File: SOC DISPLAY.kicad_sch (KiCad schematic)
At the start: 70 parts, among them IC1 CM BLE, IC2 LM5164QDDATQ1, J2 PRG, J3 OLED, U2 LP2985-3.3, U3 TPS563200, U4 STM32G0B1CBTx, U7 TJA1051T-3

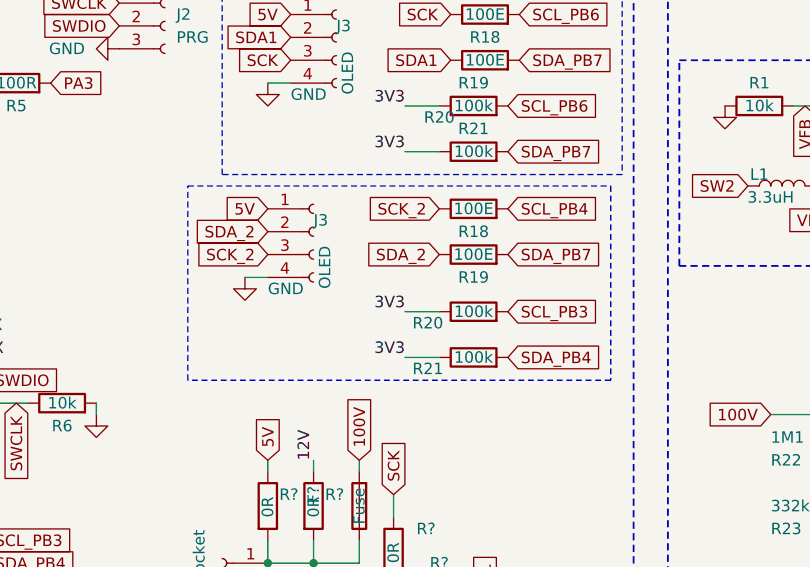
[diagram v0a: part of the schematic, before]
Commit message: Matic
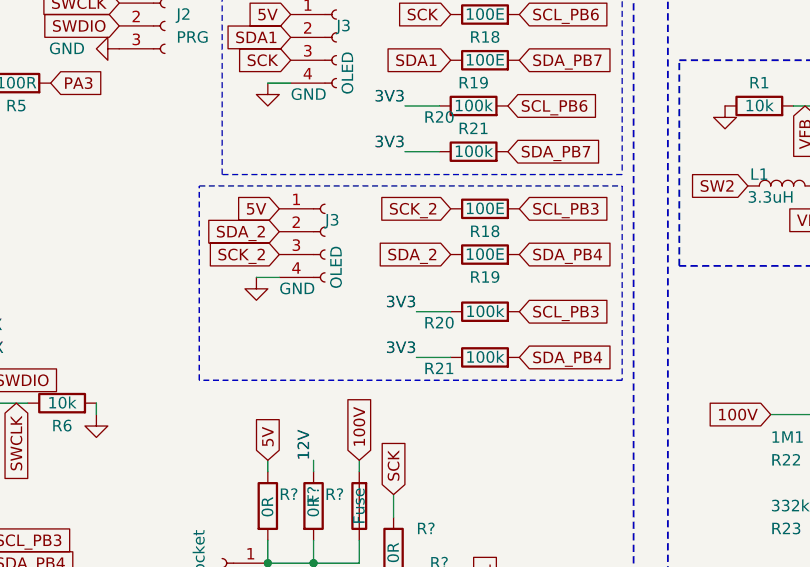
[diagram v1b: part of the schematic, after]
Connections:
- net SCL_PB4 is gone; now on net SCL_PB3: R18.2
- net SDA_PB4: now also R19.2
- net SDA_PB7: no longer R19.2
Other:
- moved on the sheet: J3, R18, R19, R20, R21

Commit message: now
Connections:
- net  SCL_PB3 is gone; now on net SCL_PB3: U4.42 (PB3)
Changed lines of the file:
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@@
     )
   )
-  (global_label " SCL_PB3" (shape input) (at 66.04 80.01 0) (fields_autoplaced)
+  (global_label "SCL_PB3" (shape input) (at 66.04 80.01 0) (fields_autoplaced)
     (effects (font (size 1.27 1.27)) (justify left))
-    (property "Intersheetrefs" "${INTERSHEET_REFS}" (at 78.1381 80.01 0)
+    (property "Intersheetrefs" "${INTERSHEET_REFS}" (at 77.1705 80.01 0)
       (effects (font (size 1.27 1.27)) (justify left) hide)
     )

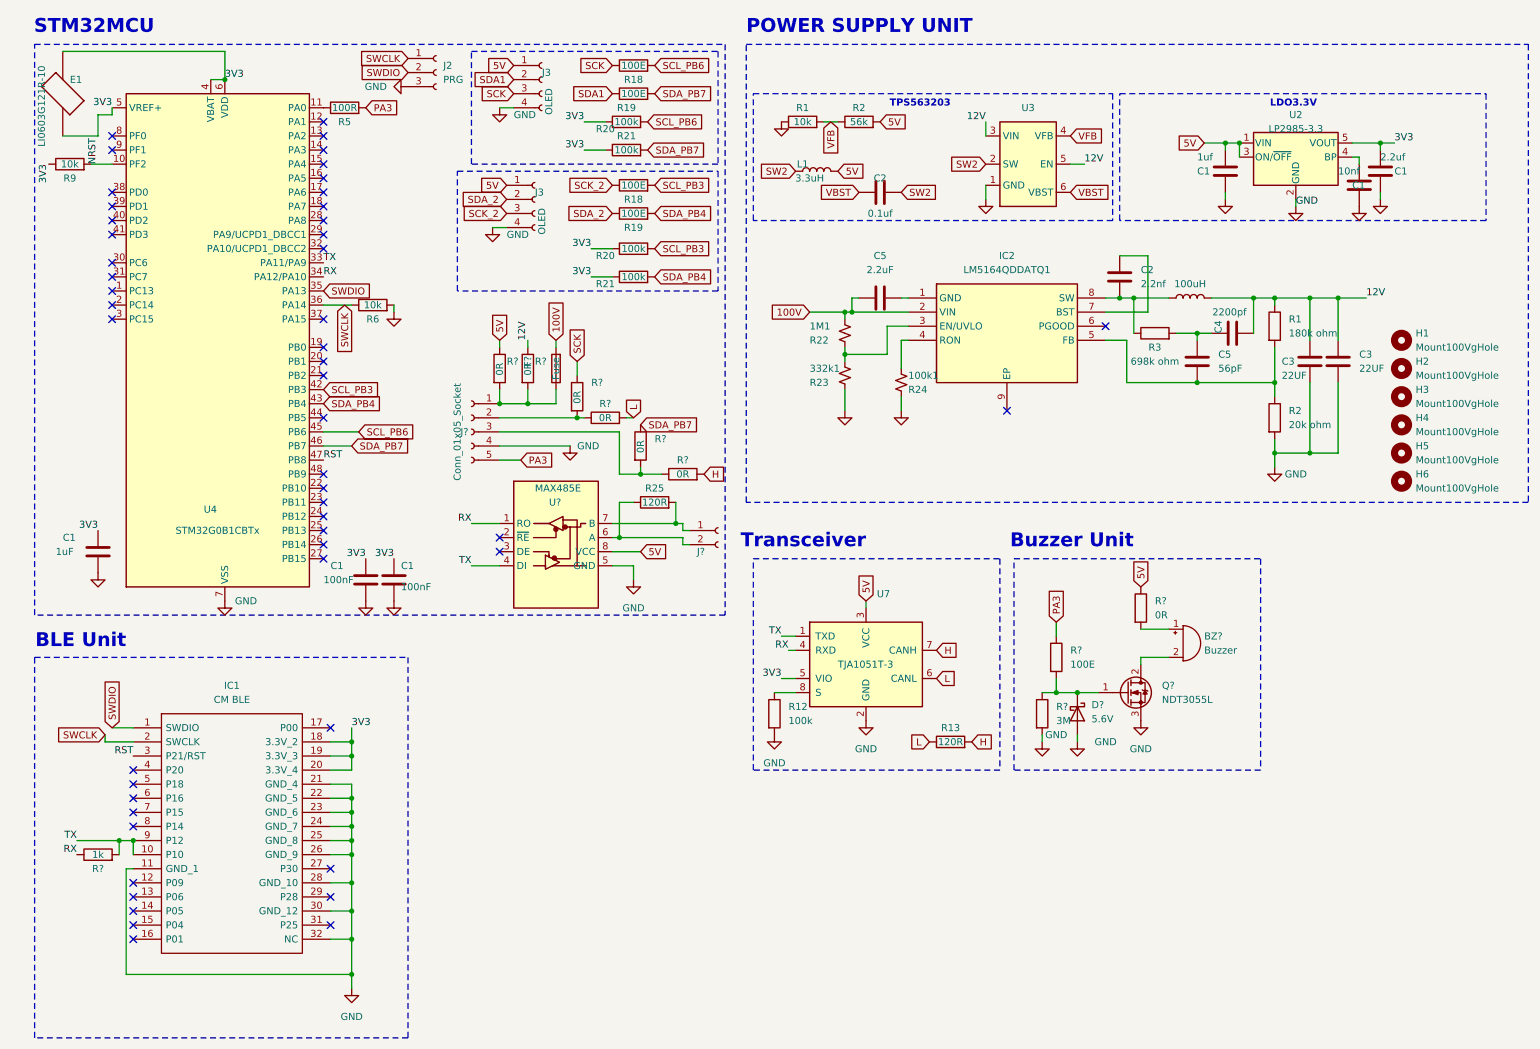
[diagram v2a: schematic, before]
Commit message: Done
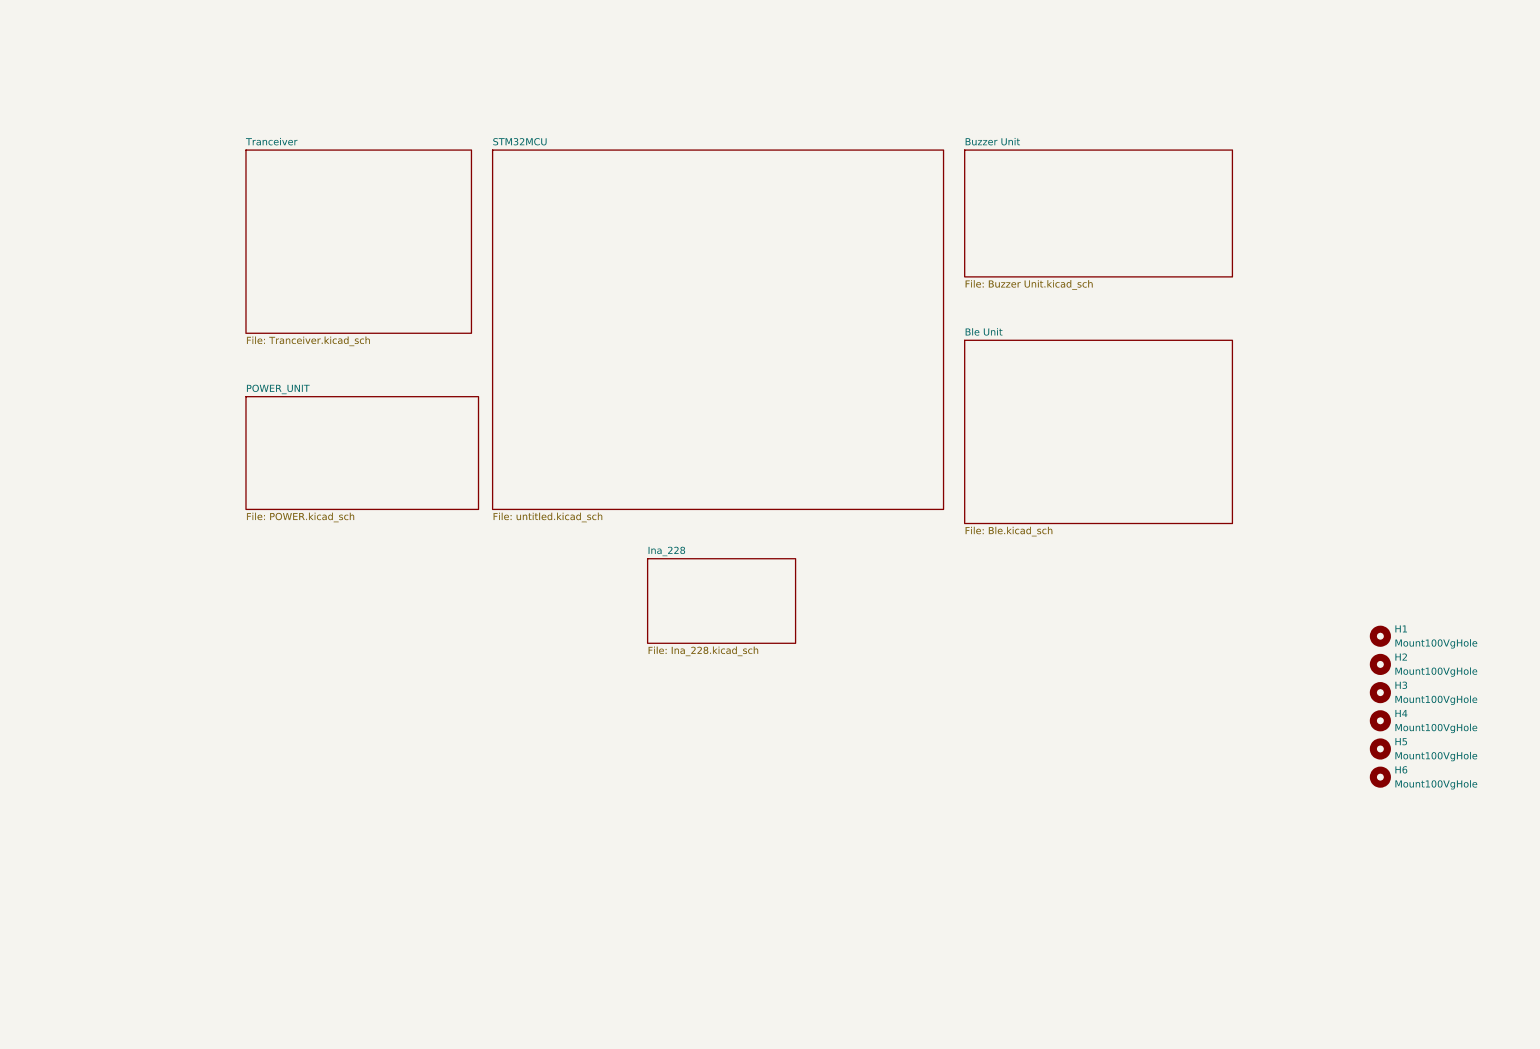
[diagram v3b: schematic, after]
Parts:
- removed 100k1: R24, Resistor_SMD:R_0603_1608Metric_Pad0.98x0.95mm_HandSolder, symbol Device:R_Small_US
- removed 1M1: R22, Resistor_SMD:R_0603_1608Metric_Pad0.98x0.95mm_HandSolder, symbol Device:R_Small_US
- removed 332k1: R23, Resistor_SMD:R_0603_1608Metric_Pad0.98x0.95mm_HandSolder, symbol Device:R_Small_US
- removed BZ?: Buzzer, Buzzer_Beeper:Indicator_PUI_AI-1440-TWT-24V-2-R, symbol Device:Buzzer
- removed C1 (x2): 100nF, Capacitor_SMD:C_0805_2012Metric_Pad1.18x1.45mm_HandSolder, symbol Device:C
- removed C1: 1uf, Capacitor_SMD:C_0805_2012Metric_Pad1.18x1.45mm_HandSolder, symbol Device:C
- removed C1: 1uF, Capacitor_SMD:C_0805_2012Metric_Pad1.18x1.45mm_HandSolder, symbol Device:C
- removed C1: 2.2uf, Capacitor_SMD:C_0805_2012Metric_Pad1.18x1.45mm_HandSolder, symbol Device:C
- removed C1: 10nf, Capacitor_SMD:C_0805_2012Metric_Pad1.18x1.45mm_HandSolder, symbol Device:C
- removed C2: 0.1uf, Capacitor_SMD:C_0805_2012Metric_Pad1.18x1.45mm_HandSolder, symbol Device:C
- removed C2: 2.2nf, Capacitor_SMD:C_0603_1608Metric_Pad1.08x0.95mm_HandSolder, symbol Device:C
- removed C3 (x2): 22UF, Capacitor_SMD:C_1206_3216Metric_Pad1.33x1.80mm_HandSolder, symbol Device:C
- removed C4: 2200pf, Capacitor_SMD:C_0805_2012Metric_Pad1.18x1.45mm_HandSolder, symbol Device:C
- removed C5: 2.2uF, Capacitor_SMD:C_0402_1005Metric_Pad0.74x0.62mm_HandSolder, symbol Device:C
- removed C5: 56pF, Capacitor_SMD:C_0402_1005Metric_Pad0.74x0.62mm_HandSolder, symbol Device:C
- removed D?: 5.6V, Diode_SMD:D_0603_1608Metric_Pad1.05x0.95mm_HandSolder, symbol Device:D_Schottky
- removed E1: LI0603G121R-10, LI0603G121R-10.kicad_mod files:FB_LI0603G121R-10, symbol LI0603G121R-10:LI0603G121R-10
- removed F?: Fuse, Fuse:Fuse_0603_1608Metric_Pad1.05x0.95mm_HandSolder, symbol Device:Fuse
- removed IC1: CM BLE, Library:CM BLE, symbol Library:COMMON_BLUETOOTH
- removed IC2: LM5164QDDATQ1, LIB_LM5164QDDATQ1.kicad_mod files:SOIC127P600X170-9N, symbol LM5164QDDATQ1:LM5164QDDATQ1
- removed J2: PRG, TerminalBlock:TerminalBlock_bornier-3_P5.08mm, symbol Connector:Conn_01x03_Socket
- removed J3 (x2): OLED, TerminalBlock:TerminalBlock_bornier-4_P5.08mm, symbol Connector:Conn_01x04_Socket
- removed J?: Conn_01x05_Socket, Connector_JST:JST_PH_S5B-PH-K_1x05_P2.00mm_Horizontal, symbol Connector:Conn_01x05_Socket
- removed J?: Conn_01x02_Socket, TerminalBlock:TerminalBlock_bornier-2_P5.08mm, symbol Connector:Conn_01x02_Socket
- removed L1: 100uH, Inductor_SMD:L_0805_2012Metric_Pad1.15x1.40mm_HandSolder, symbol Device:L
- removed L1: 3.3uH, Inductor_SMD:L_0402_1005Metric_Pad0.77x0.64mm_HandSolder, symbol Device:L
- removed Q?: NDT3055L, Package_TO_SOT_SMD:SOT-223-3_TabPin2, symbol Transistor_FET:NDT3055L
- removed R1, R6, R9: 10k, Resistor_SMD:R_0603_1608Metric_Pad0.98x0.95mm_HandSolder, symbol Device:R
- removed R1: 180k ohm, Resistor_SMD:R_0603_1608Metric_Pad0.98x0.95mm_HandSolder, symbol Device:R
- removed R12, R20 (x2), R21 (x2): 100k, Resistor_SMD:R_0603_1608Metric_Pad0.98x0.95mm_HandSolder, symbol Device:R
- removed R13, R25: 120R, Resistor_SMD:R_0603_1608Metric_Pad0.98x0.95mm_HandSolder, symbol Device:R
- removed R18 (x2), R19 (x2), R?: 100E, Resistor_SMD:R_0603_1608Metric_Pad0.98x0.95mm_HandSolder, symbol Device:R
- removed R2: 20k ohm, Resistor_SMD:R_0603_1608Metric_Pad0.98x0.95mm_HandSolder, symbol Device:R
- removed R2: 56k, Resistor_SMD:R_0603_1608Metric_Pad0.98x0.95mm_HandSolder, symbol Device:R
- removed R3: 698k ohm, Resistor_SMD:R_0603_1608Metric_Pad0.98x0.95mm_HandSolder, symbol Device:R
- removed R5: 100R, Resistor_SMD:R_0603_1608Metric_Pad0.98x0.95mm_HandSolder, symbol Device:R
- removed R?: 3M, Resistor_SMD:R_0603_1608Metric_Pad0.98x0.95mm_HandSolder, symbol Device:R
- removed R? (x7): 0R, Resistor_SMD:R_0603_1608Metric_Pad0.98x0.95mm_HandSolder, symbol Device:R
- removed R?: 1k, Resistor_SMD:R_0603_1608Metric_Pad0.98x0.95mm_HandSolder, symbol Device:R
- removed U2: LP2985-3.3, Package_TO_SOT_SMD:SOT-23-5, symbol Regulator_Linear:LP2985-3.3
- removed U3: TPS563200, Package_TO_SOT_SMD:SOT-23-6, symbol Regulator_Switching:TPS563200
- removed U4: STM32G0B1CBTx, Package_QFP:LQFP-48_7x7mm_P0.5mm, symbol MCU_ST_STM32G0:STM32G0B1CBTx
- removed U7: TJA1051T-3, Package_SO:SOIC-8_3.9x4.9mm_P1.27mm, symbol Interface_CAN_LIN:TJA1051T-3
- removed U?: MAX485E, MAX485ESA_T.kicad_mod files:SOIC127P600X175-8N, symbol Interface_UART:MAX485E
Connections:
- no-connect marks 51 -> 0
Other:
- added sheet Ble Unit (Ble.kicad_sch)
- added sheet Buzzer Unit  (Buzzer Unit.kicad_sch)
- added sheet Ina_228 (Ina_228.kicad_sch)
- added sheet POWER_UNIT (POWER.kicad_sch)
- added sheet STM32MCU (untitled.kicad_sch)
- added sheet Tranceiver (Tranceiver.kicad_sch)
- note removed: "BLE Unit"
- note removed: "Buzzer Unit"
- note removed: "LDO3.3V"
- note removed: "POWER SUPPLY UNIT"
- note removed: "STM32MCU"
- note removed: "TPS563203"
- note removed: "Transceiver"
- moved on the sheet: H1, H2, H3, H4, H5, H6
